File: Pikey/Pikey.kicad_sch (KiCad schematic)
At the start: 68 parts, among them J1 DX07P024AJ1R1500, J2 Conn_01x03, J3 Microsd card, SW1 CK_KMS2xxG, SW2 CK_KMS2xxG, U1 RP2350B, U2 NCP1117-3.3_SOT223, U3 W25Q128JVS, U4 nRF8001, U5 BAL-NRF01D3, Y1 ABM8-272-T3, Y2 ABS05-32.768KHZ-T, Y3 ABM8-16.000MHZ-B2-T

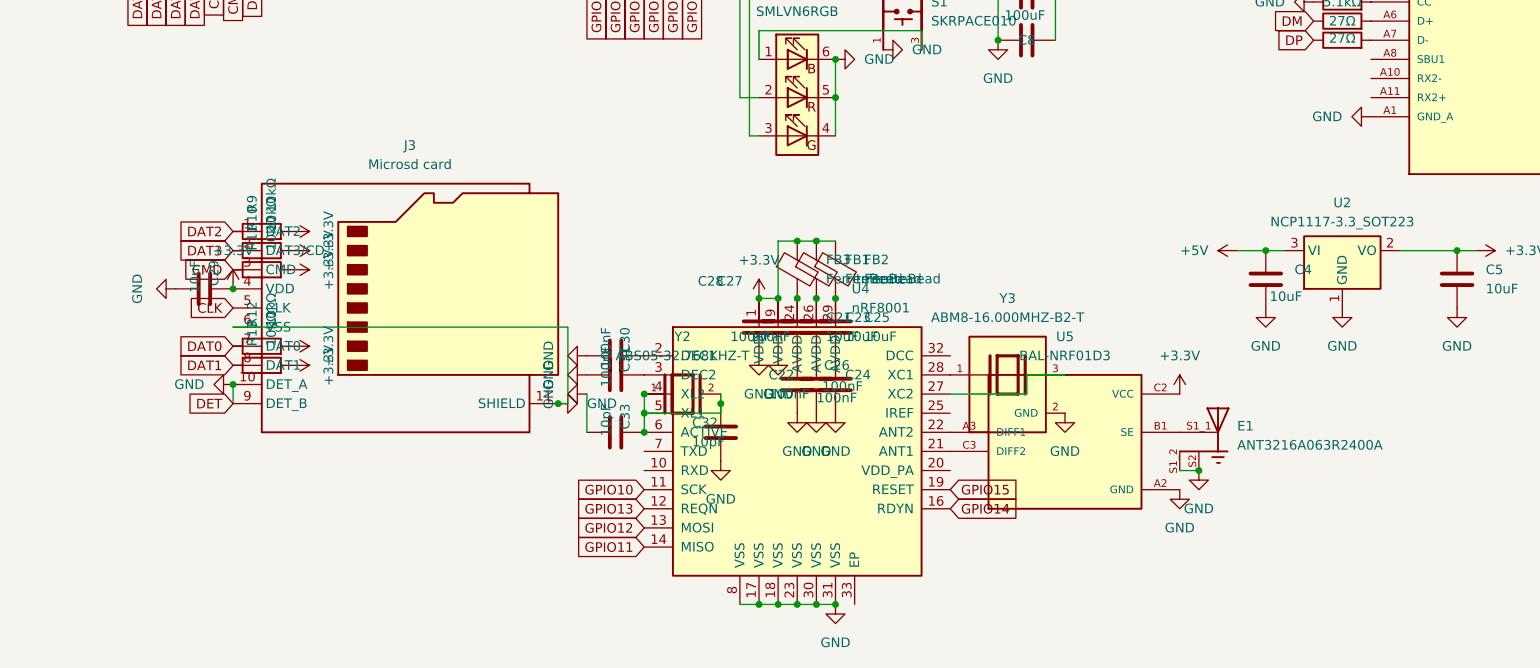
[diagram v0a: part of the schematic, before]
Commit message: 20th april update
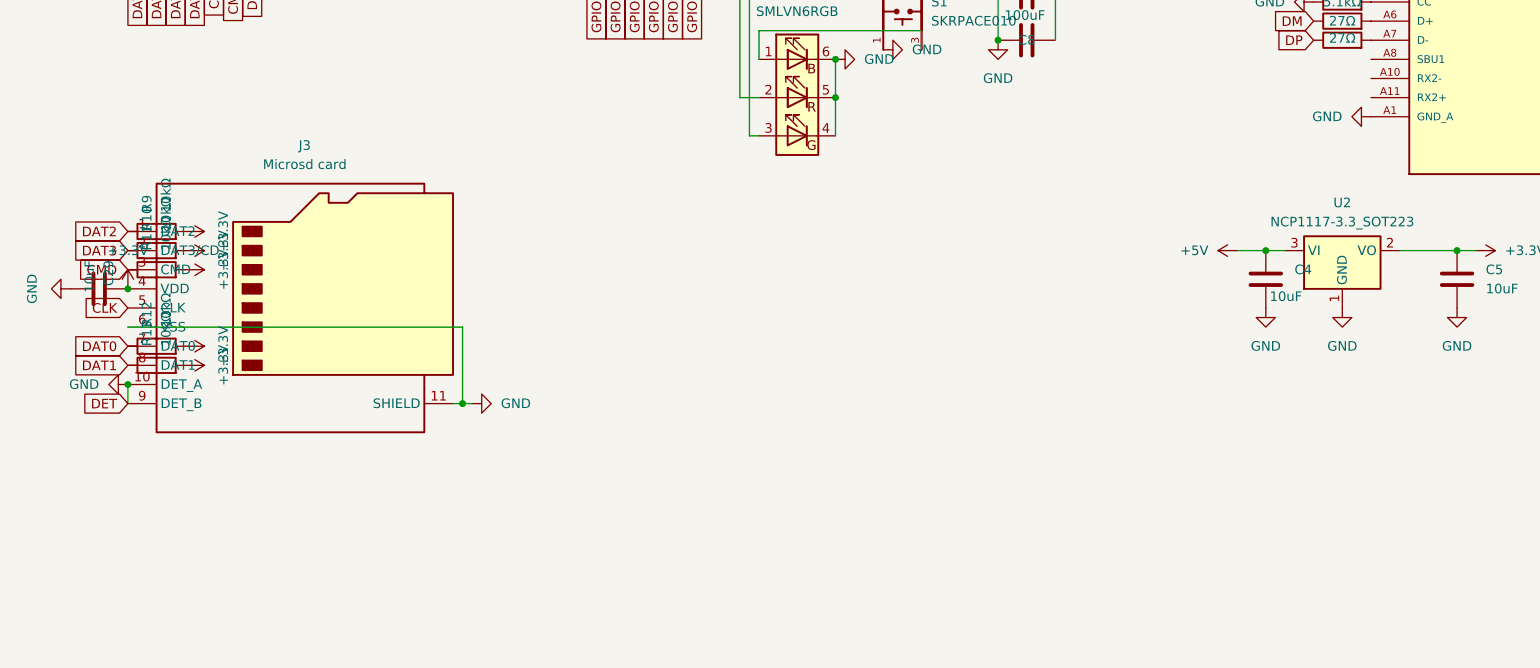
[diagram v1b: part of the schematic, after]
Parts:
- removed C21, C23, C25: 10uF, Capacitor_SMD:C_0402_1005Metric, symbol Device:C
- removed C22, C24, C26, C27, C28, C30, C31: 100nF, Capacitor_SMD:C_0402_1005Metric, symbol Device:C
- removed C32, C33: 10pF, Capacitor_SMD:C_0402_1005Metric, symbol Device:C
- removed E1: ANT3216A063R2400A, ANT3216A063R2400A:XDCR_ANT3216A063R2400A, symbol ANT3216A063R2400A:ANT3216A063R2400A
- removed FB1, FB2, FB3: FerriteBead, Inductor_SMD:L_0402_1005Metric, symbol Device:FerriteBead
- removed U4: nRF8001, Package_DFN_QFN:QFN-32-1EP_5x5mm_P0.5mm_EP3.45x3.45mm, symbol RF_Bluetooth:nRF8001
- removed U5: BAL-NRF01D3, BAL-NRF01D3:IC_BAL-NRF01D3, symbol BAL-NRF01D3:BAL-NRF01D3
- removed Y2: ABS05-32.768KHZ-T, ABS05-32.768KHZ-T:XTAL_ABS05-32.768KHZ-T, symbol ABS05-32.768KHZ-T:ABS05-32.768KHZ-T
- removed Y3: ABM8-16.000MHZ-B2-T, ABM8-16.000MHZ-B2-T:XTAL_ABM8-16.000MHZ-B2-T, symbol ABM8-16.000MHZ-B2-T:ABM8-16.000MHZ-B2-T
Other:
- moved on the sheet: C29, J3, R10, R11, R12, R13, R9

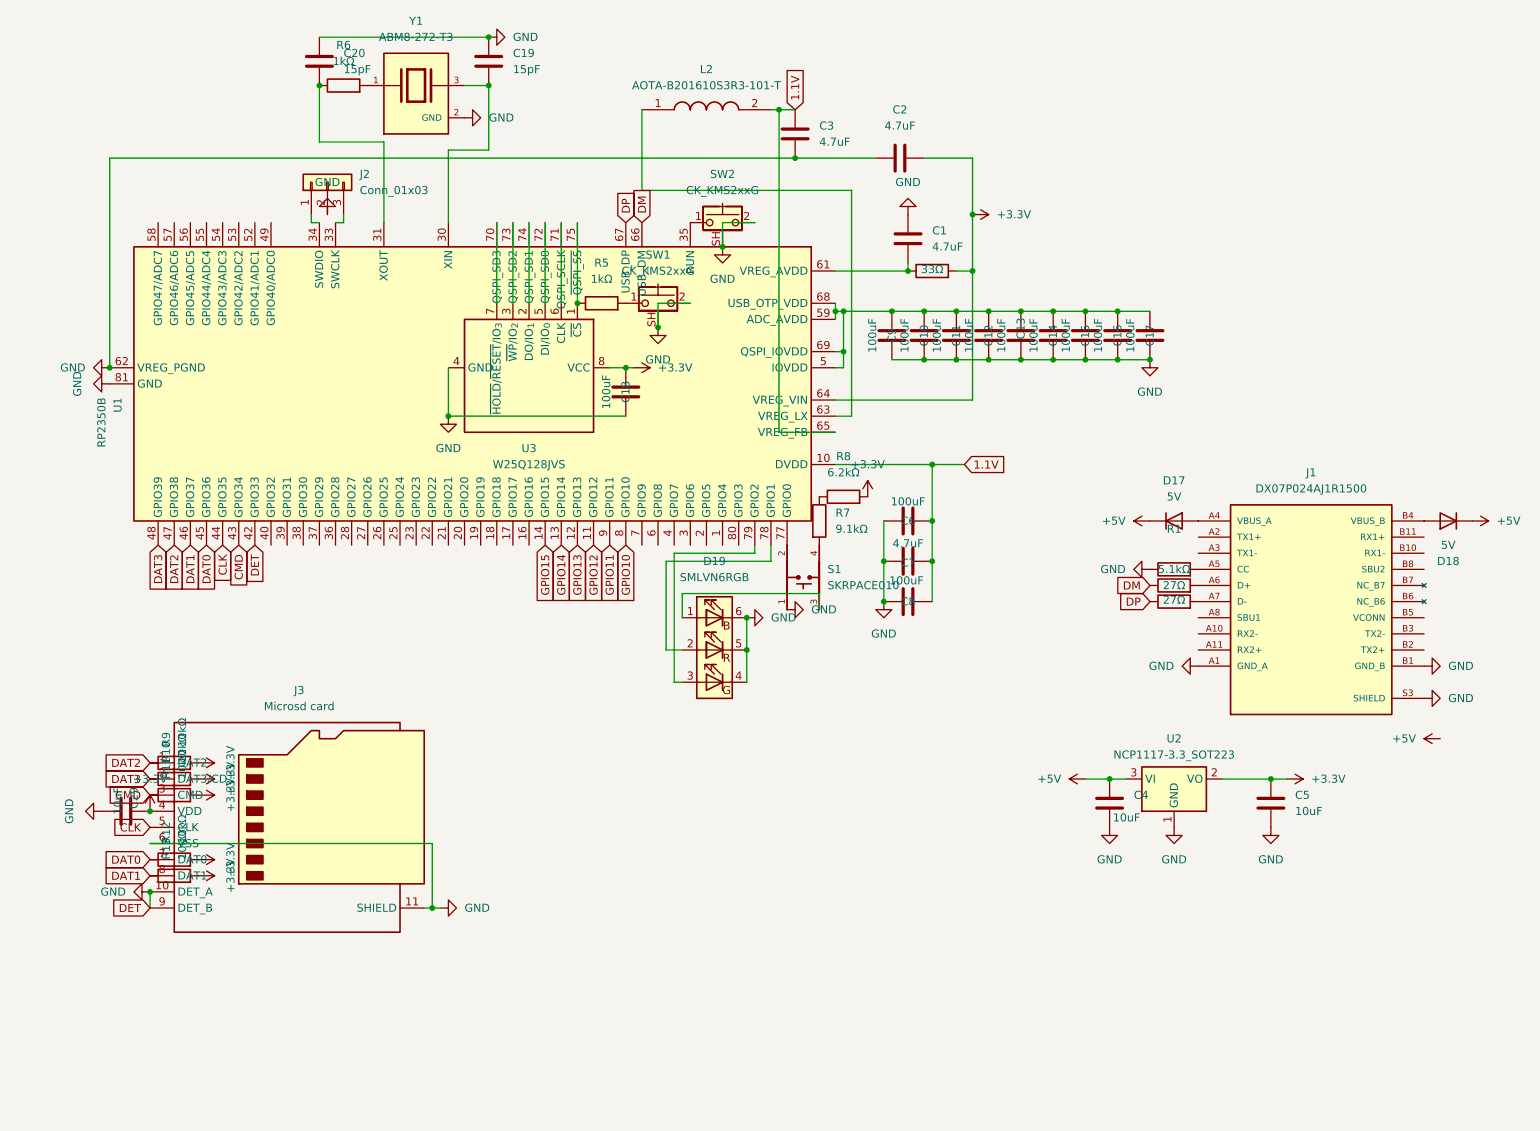
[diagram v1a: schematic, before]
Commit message: May 2nd update
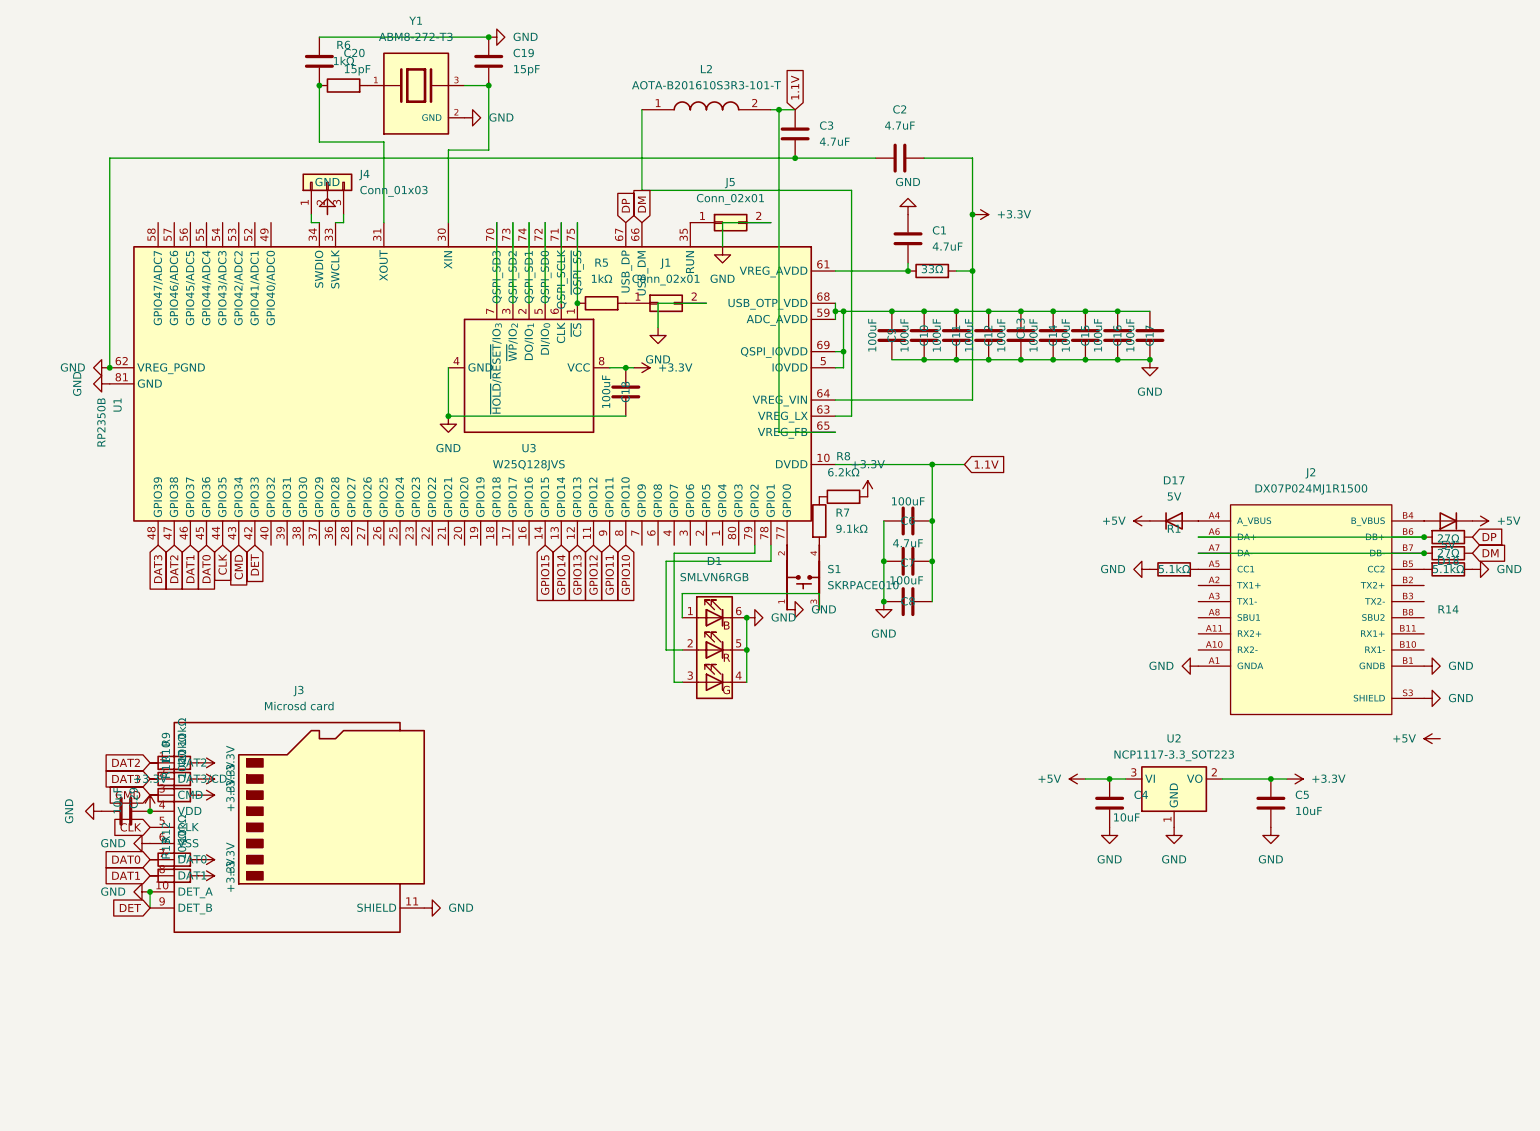
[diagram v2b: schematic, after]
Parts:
- removed D19: SMLVN6RGB, LED_SMD:LED_2010_5025Metric, symbol LED:SMLVN6RGB
- removed J1: DX07P024AJ1R1500, DX07P024AJ1R1500:JAE_DX07P024AJ1R1500, symbol DX07P024AJ1R1500:DX07P024AJ1R1500
- removed SW1, SW2: CK_KMS2xxG, Button_Switch_SMD:SW_SPST_CK_KMS2xxGP, symbol Switch:CK_KMS2xxG
- added D1: SMLVN6RGB, LED_SMD:LED_ROHM_SMLVN6, symbol LED:SMLVN6RGB
- added J1, J5: Conn_02x01, Connector_PinHeader_1.00mm:PinHeader_2x01_P1.00mm_Vertical, symbol Connector_Generic:Conn_02x01
- added J2: DX07P024MJ1R1500, DX07P024MJ1R1500:JAE_DX07P024MJ1R1500, symbol DX07P024MJ1R1500:DX07P024MJ1R1500
- added R14: 5.1kΩ, Resistor_SMD:R_0201_0603Metric, symbol Device:R
- J4: renamed from J2; footprint Connector_PinHeader_1.00mm:PinHeader_1x03_P1.00mm_Vertical_SMD -> Connector_PinHeader_1.00mm:PinHeader_1x03_P1.00mm_Vertical
- L2: footprint AOTAB201610S3R3101T -> AOTA-B201610S3R3-101-T:AOTAB201610S3R3101T
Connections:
- net GND: now also D1.4 (GK), D1.5 (RK), D1.6 (BK), J1.2 (Pin_2), J2.A1 (GNDA), J2.A12 (GNDA), J2.B1 (GNDB), J2.B12 (GNDB), J2.S3 (SHIELD), J2.S4 (SHIELD), J2.S5 (SHIELD), J2.S6 (SHIELD), J5.2 (Pin_2), R14.1
- net at U1.35 (RUN): now also J5.1 (Pin_1)
- net at S1.3: now also D1.1 (BA)
- net at U1.78 (GPIO1): now also D1.2 (RA)
- net at U1.79 (GPIO2): now also D1.3 (GA)
- net at R1.2: now also J2.A5 (CC1)
- net at R2.2: now also J2.A7 (DA-), J2.B7 (DB-)
- net at R3.2: now also J2.A6 (DA+), J2.B6 (DB+)
- net at R5.2: now also J1.1 (Pin_1)
- net VBUS_A renamed A_VBUS
- net A_VBUS: now also J2.A4 (A_VBUS), J2.A9 (A_VBUS)
- net VBUS_B renamed B_VBUS
- net B_VBUS: now also J2.B4 (B_VBUS), J2.B9 (B_VBUS)
- new net: J2.B5 (CC2), R14.2

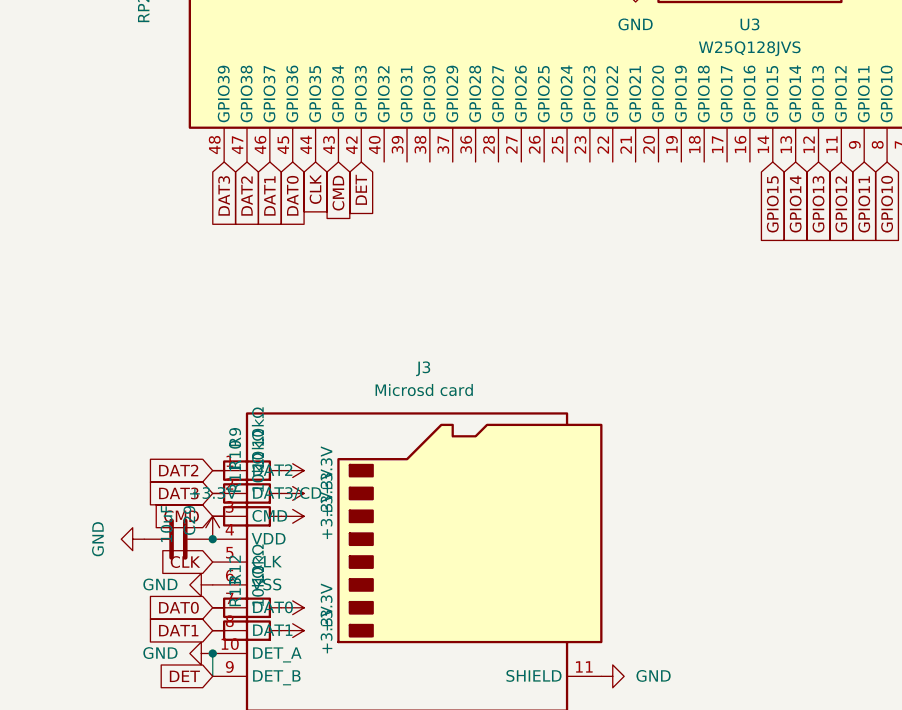
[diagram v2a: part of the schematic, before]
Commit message: Monday 4th May update
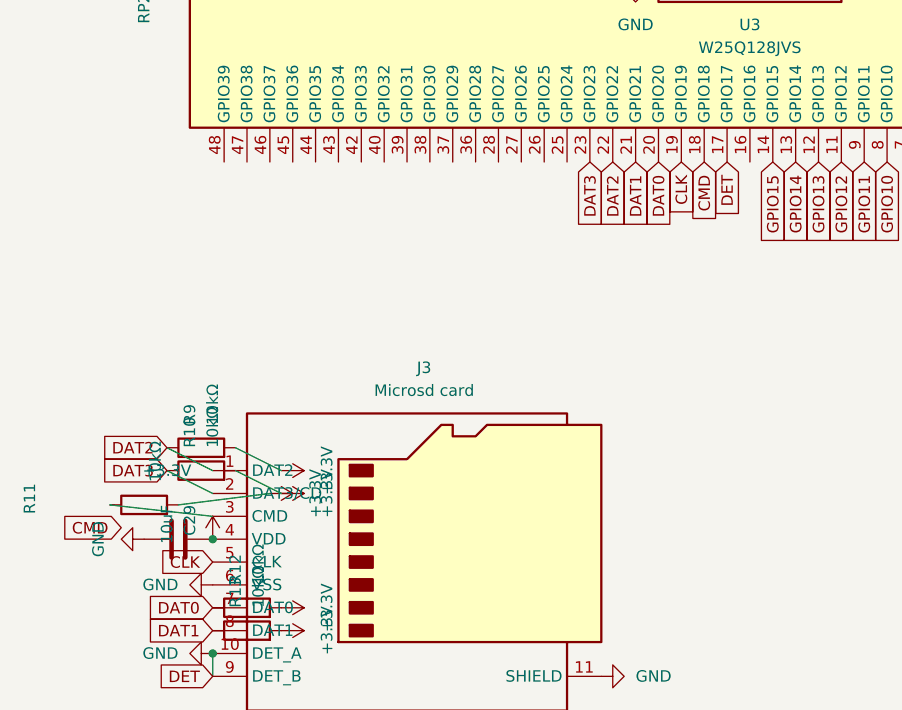
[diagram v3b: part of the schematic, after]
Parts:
- D1: LCSC Part number (none) -> C2909770; Name (none) -> ROHM SMLVN6RGB1U1
- J1, J5: now left out of the parts list
- J2: LCSC Part number (none) -> C134112; Name (none) -> JAE Electronics DX07P024MJ1R1500
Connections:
- net CLK: now also U1.19 (GPIO19); no longer U1.44 (GPIO35)
- net CMD: now also U1.18 (GPIO18); no longer J3.3 (CMD), R11.1, U1.43 (GPIO34)
- net DAT0: now also U1.20 (GPIO20); no longer U1.45 (GPIO36)
- net DAT1: now also U1.21 (GPIO21); no longer U1.46 (GPIO37)
- net DAT2: now also U1.22 (GPIO22); no longer U1.47 (GPIO38)
- net DAT3: now also U1.23 (GPIO23); no longer U1.48 (GPIO39)
- net GND: now also U1.17 (GPIO17); no longer U1.42 (GPIO33)
- new net: J3.3 (CMD), R11.1
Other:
- moved on the sheet: R10, R11, R9
